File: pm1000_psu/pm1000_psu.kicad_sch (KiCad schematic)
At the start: 42 parts, among them J1 Screw_Terminal_01x05, U1 LM317_TO-220, U2 LM317_TO-220, U3 LM317_TO-220

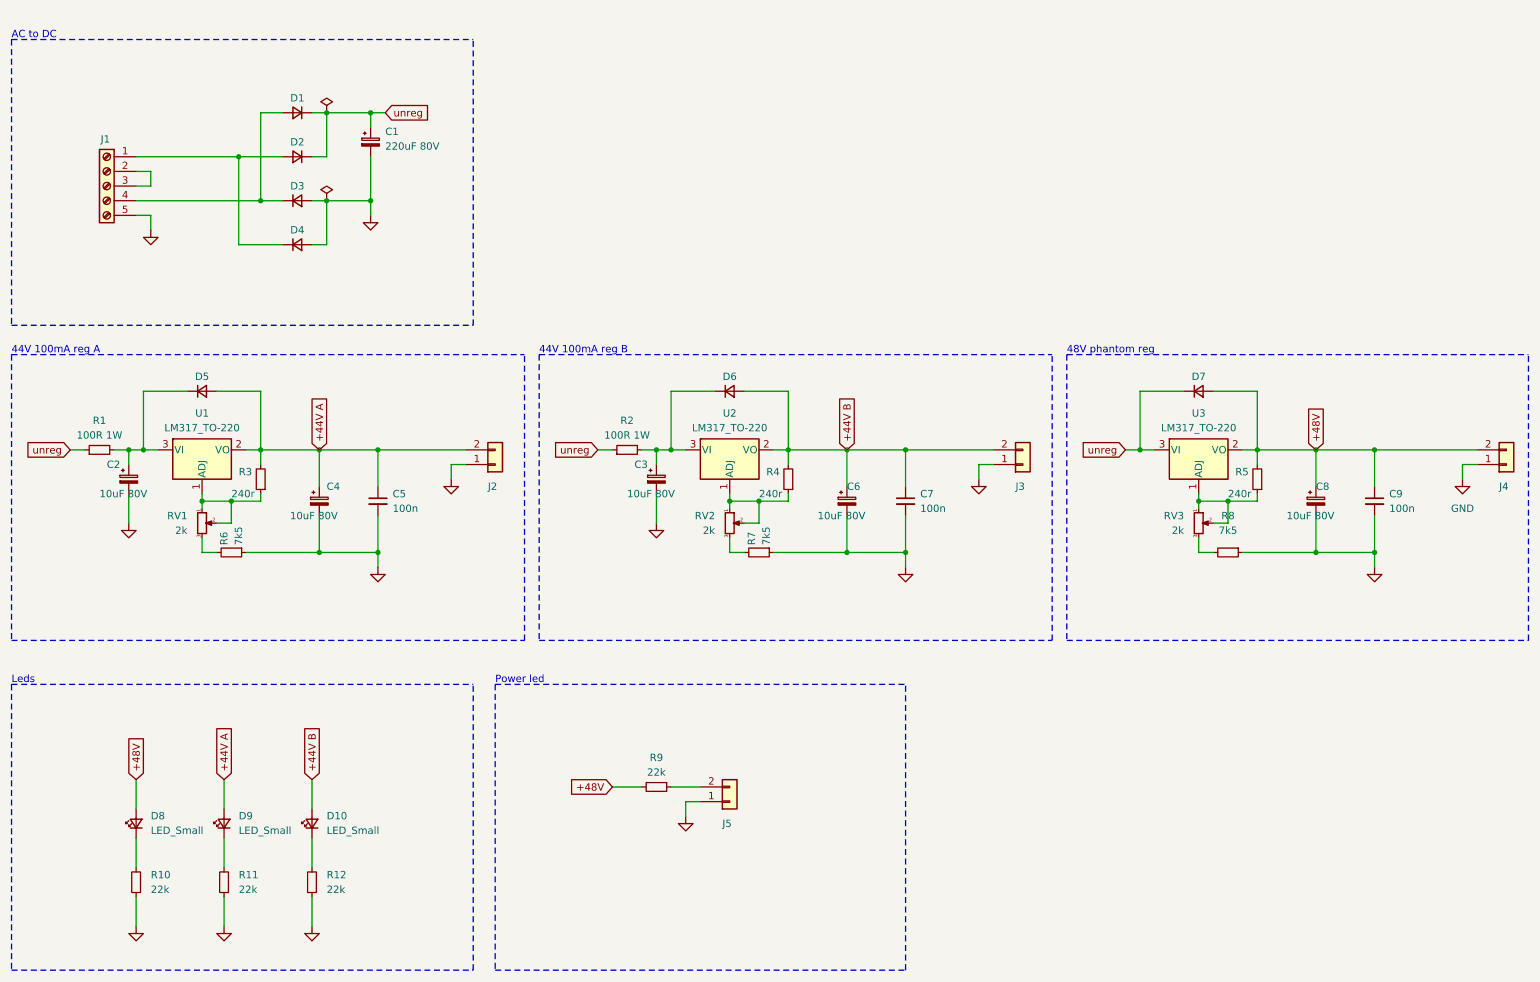
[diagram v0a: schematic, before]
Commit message: re-engineer psu board
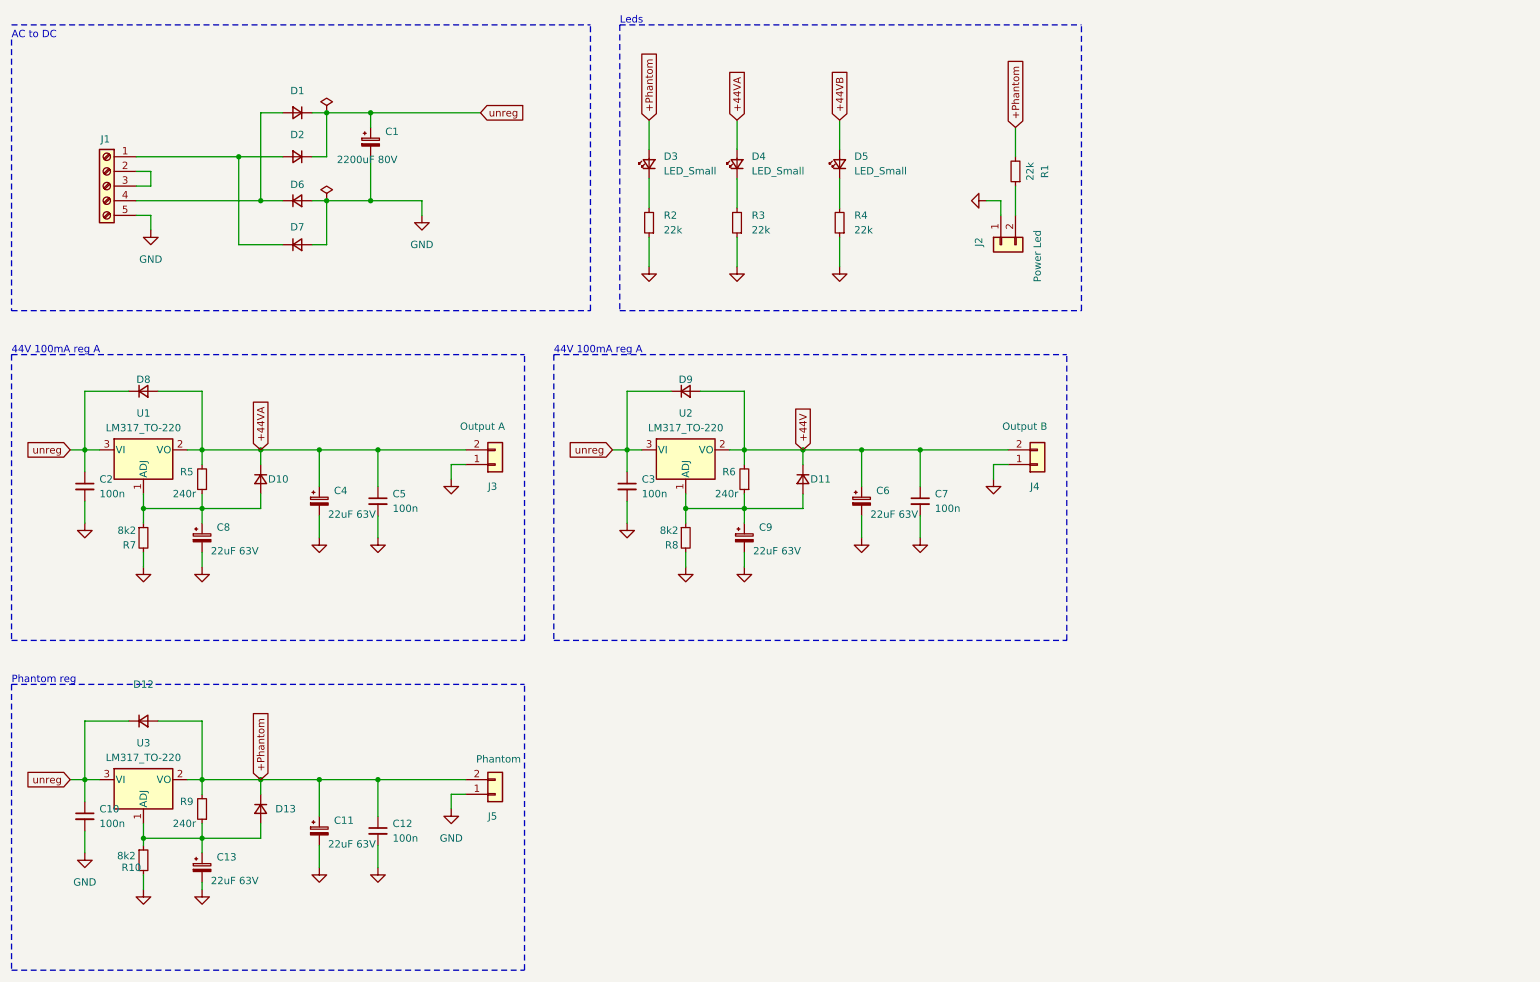
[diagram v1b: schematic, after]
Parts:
- removed C2, C3: 10uF 80V, Capacitor_THT:CP_Radial_D6.3mm_P2.50mm, symbol Device:C_Polarized_Small
- removed D10: LED_Small, LED_THT:LED_D3.0mm, symbol Device:LED_Small
- removed D3, D4, D5: 1n4004, Diode_THT:D_DO-41_SOD81_P10.16mm_Horizontal, symbol Device:D_Small
- removed J3: ~, Connector_Molex:Molex_KK-396_5273-02A_1x02_P3.96mm_Vertical, symbol Connector_Generic:Conn_01x02
- removed R1, R2: 100R 1W, Resistor_THT:R_Axial_DIN0411_L9.9mm_D3.6mm_P15.24mm_Horizontal, symbol Device:R_Small
- removed R12: 22k, Resistor_THT:R_Axial_DIN0207_L6.3mm_D2.5mm_P10.16mm_Horizontal, symbol Device:R_Small
- removed R7: 7k5, Resistor_THT:R_Axial_DIN0207_L6.3mm_D2.5mm_P10.16mm_Horizontal, symbol Device:R_Small
- removed RV1, RV2, RV3: 2k, Potentiometer_THT:Potentiometer_Piher_PT-10-V05_Vertical, symbol Device:R_Potentiometer_Small
- added C10, C2, C3: 100n, Capacitor_THT:C_Disc_D5.0mm_W2.5mm_P2.50mm, symbol Device:C_Small
- added C11, C13, C9: 22uF 63V, Capacitor_THT:CP_Radial_D8.0mm_P3.50mm, symbol Device:C_Polarized_Small
- added D10, D11, D12, D13, D8, D9: D_Small, Diode_THT:D_DO-41_SOD81_P10.16mm_Horizontal, symbol Device:D_Small
- added D5: LED_Small, LED_THT:LED_D3.0mm, symbol Device:LED_Small
- added J4: Output B, Connector_Molex:Molex_KK-396_5273-02A_1x02_P3.96mm_Vertical, symbol Connector_Generic:Conn_01x02
- added R6: 240r, Resistor_THT:R_Axial_DIN0207_L6.3mm_D2.5mm_P10.16mm_Horizontal, symbol Device:R_Small
- added R8: 8k2, Resistor_THT:R_Axial_DIN0207_L6.3mm_D2.5mm_P10.16mm_Horizontal, symbol Device:R_Small
- C1: value 220uF 80V -> 2200uF 80V; footprint Capacitor_THT:CP_Radial_D12.5mm_P5.00mm -> Capacitor_THT:CP_Radial_D22.0mm_P10.00mm_SnapIn
- C4, C6, C8: value 10uF 80V -> 22uF 63V; footprint Capacitor_THT:CP_Radial_D6.3mm_P2.50mm -> Capacitor_THT:CP_Radial_D8.0mm_P3.50mm; Mouser # 667-ECA-2AM100I -> 667-ECA-2AHG221B
- D1, D2, D6, D7: value 1n4004 -> D_Small; Mouser # 621-1N4007 -> (none)
- J2: renamed from J5; value ~ -> Power Led
- J3: renamed from J2; value ~ -> Output A
- J5: renamed from J4; value ~ -> Phantom
- R10: renamed from R8; value 7k5 -> 8k2
- R4: value 240r -> 22k; Mouser # 603-MFR-25FRF52-240R -> 603-MFR-25FRF52-2K2
- R7: renamed from R6; value 7k5 -> 8k2
- renumbered C9 to C12, D8 to D3, D9 to D4, R9 to R1, R10 to R2, R11 to R3, R3 to R5, R5 to R9
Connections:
- net GND: now also D6.2 (A), D7.2 (A), R10.2, R4.1, R7.2, C10.2, C11.2, C13.2, C2.2, C3.2, C9.2, J4.1 (Pin_1), R8.2; no longer R10.1, R7.1
- net unreg: now also U1.3 (VI), U2.3 (VI), C10.1, C2.1, C3.1, D12.1 (K), D8.1 (K), D9.1 (K); no longer D7.1 (K)
- net at R5.1, U1.1 (ADJ): now also C8.1, R7.1, D10.2 (A)
- net at U2.1 (ADJ): now also C9.1, D11.2 (A), R6.1, R8.1; no longer R4.1
- net at D6.1 (K): now also D1.2 (A), J1.4 (Pin_4); no longer U2.3 (VI)
- net at D2.2 (A), J1.1 (Pin_1): now also D7.1 (K)
- net at R9.1, U3.1 (ADJ): now also R10.1, C13.1, D13.2 (A)
- net +44V A renamed +44VA
- net +44VA: now also D10.1 (K), D8.2 (A)
- net +44V B renamed +44V
- net +44V: now also D11.1 (K), D9.2 (A), J4.2 (Pin_2), R6.2; no longer D6.2 (A), R4.2
- net +48V renamed +Phantom
- net +Phantom: now also C11.1, D12.2 (A), D13.1 (K); no longer C8.1, D7.2 (A)
- new net: D5.1 (K), R4.2
- new net +44VB: D5.2 (A)
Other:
- note added: "Phantom reg"
- note removed: "44V 100mA reg B"
- note removed: "48V phantom reg"
- note removed: "Power led"
- moved on the sheet: C12, D3, D4, J2, J5, R1, R10, R2, R3, R5, R7, R9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
